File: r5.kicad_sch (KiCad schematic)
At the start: 80 parts, among them SW10 SW_SPDT, SW60 SW_SPDT, SW70 SW_SPDT, SW80 SW_SPDT, U10 LMZ22005, U20 DRV8871DDA, U21 DRV8871DDA, U22 DRV8871DDA, U23 DRV8871DDA, U24 DRV8871DDA, U25 DRV8871DDA, U50 PI22, U60 PCA9685PW, U70 74HC540, U71 74HC540, U80 Pico, X10 Conn_01x02, X11 Conn_01x02, X12 Conn_01x02, X20 Conn_01x06, X21 Conn_01x06, X22 Conn_01x06, X23 Conn_01x06, X24 Conn_01x06, X25 Conn_01x06, X40 Conn_01x04, X90 3X3HEADER, X91 4X3HEADER, X92 SDD1309, X93 GY-BNO08X

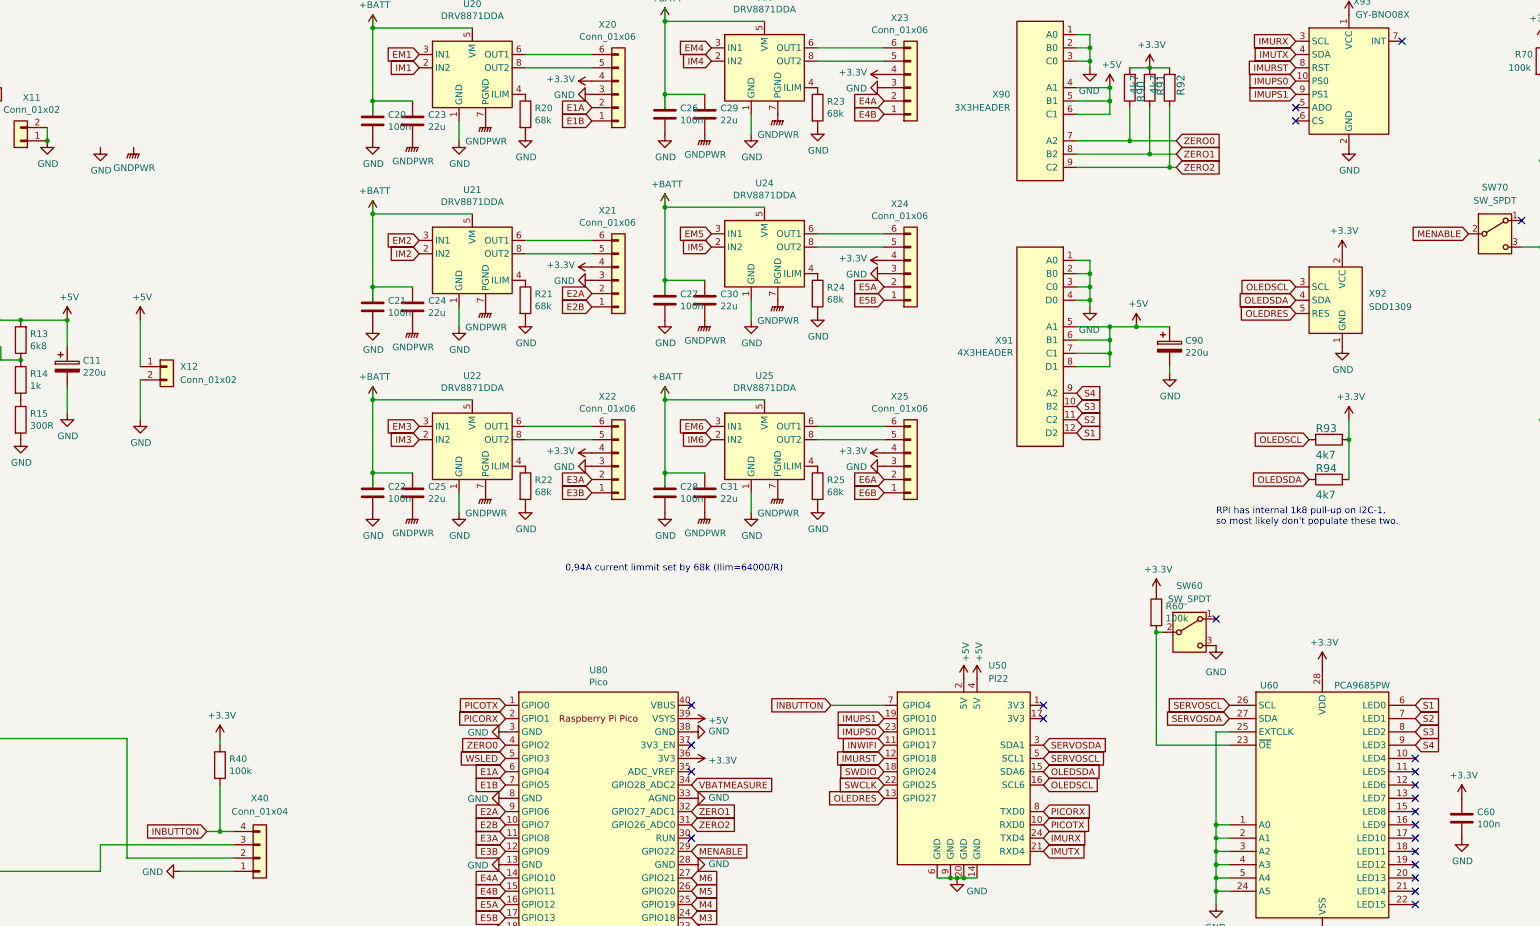
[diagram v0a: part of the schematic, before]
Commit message: routing continued
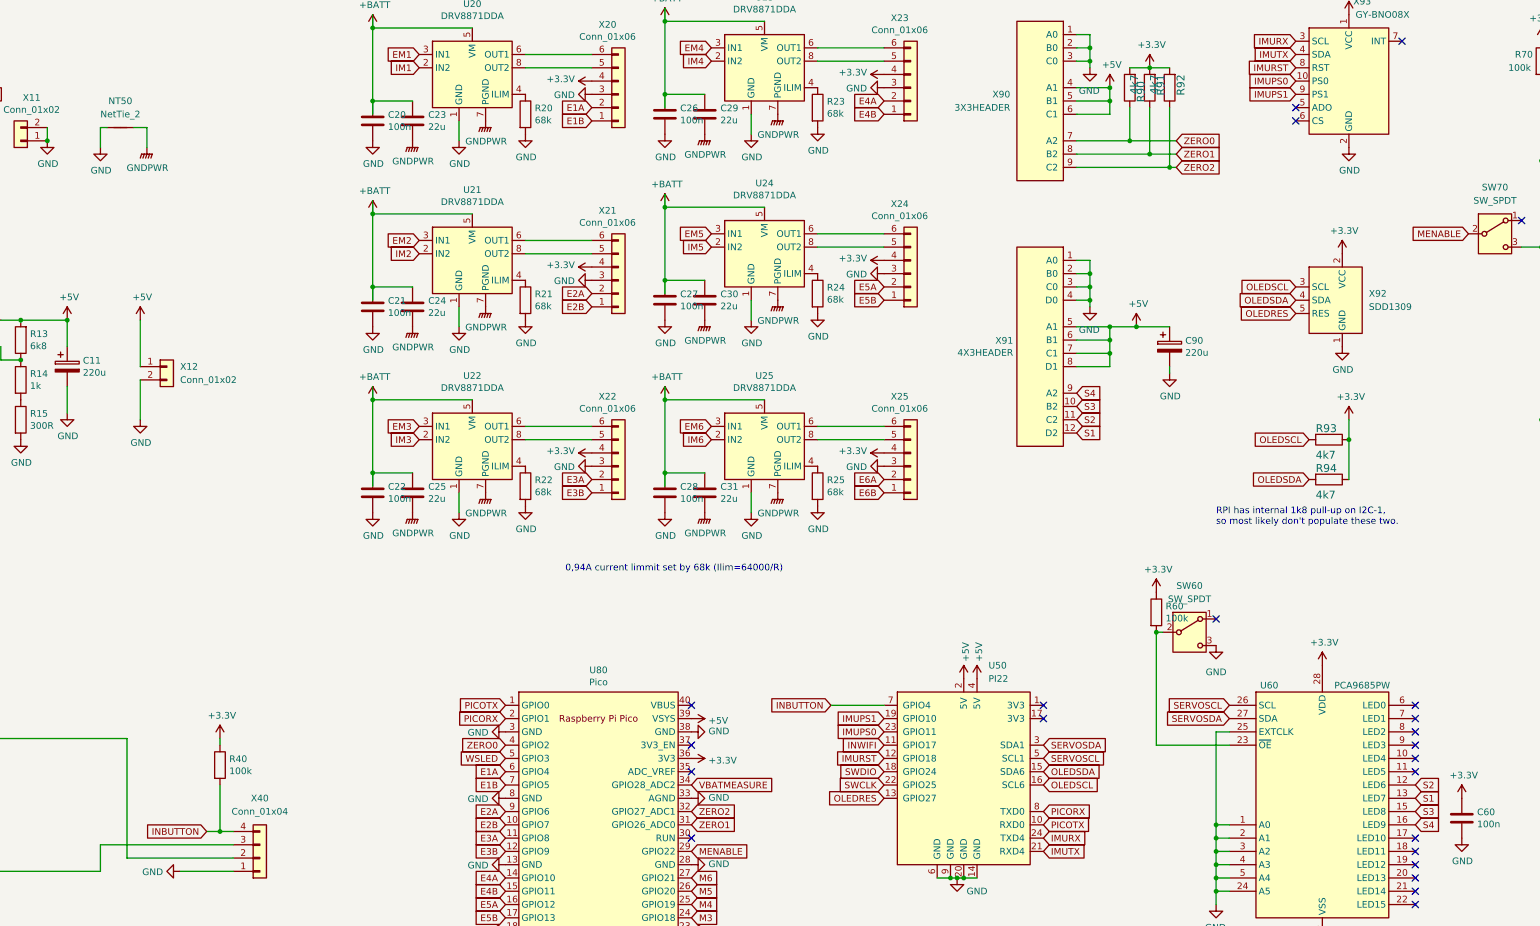
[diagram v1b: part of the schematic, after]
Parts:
- added NT50: NetTie_2, NetTie:NetTie-2_SMD_Pad2.0mm, symbol Device:NetTie_2
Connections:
- net GND: now also NT50.1
- net GNDPWR: now also NT50.2
- net S1: now also U60.13 (LED7); no longer U60.6 (LED0)
- net S2: now also U60.12 (LED6); no longer U60.7 (LED1)
- net S3: now also U60.15 (LED8); no longer U60.8 (LED2)
- net S4: now also U60.16 (LED9); no longer U60.9 (LED3)
- net ZERO1: now also U80.31 (GPIO26_ADC0); no longer U80.32 (GPIO27_ADC1)
- net ZERO2: now also U80.32 (GPIO27_ADC1); no longer U80.31 (GPIO26_ADC0)
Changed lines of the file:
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@@
   )
   (no_connect (at 278.13 175.26))
-  (no_connect (at 349.25 193.04))
+  (no_connect (at 349.25 177.8))
   (no_connect (at 58.42 109.22))
   (no_connect (at 410.21 58.42))
-  (no_connect (at 349.25 190.5))
+  (no_connect (at 349.25 172.72))
   (no_connect (at 210.82 185.42))
   (no_connect (at 349.25 200.66))
@@
   (no_connect (at 326.39 60.96))
   (no_connect (at 410.21 60.96))
-  (no_connect (at 349.25 187.96))
+  (no_connect (at 349.25 175.26))
   (no_connect (at 349.25 205.74))
   (no_connect (at 410.21 113.03))
@@
   (no_connect (at 45.72 107.95))
   (no_connect (at 210.82 198.12))
-  (no_connect (at 349.25 195.58))
+  (no_connect (at 349.25 180.34))
   (no_connect (at 349.25 210.82))
   (no_connect (at 326.39 58.42))
@@
     (stroke (width 0) (type default))
   )
+  (wire (pts (xy 97.79 62.23) (xy 99.06 62.23))
+    (stroke (width 0) (type default))
+  )
   (wire (pts (xy 294.64 50.8) (xy 298.45 50.8))
     (stroke (width 0) (type default))
@@
     (stroke (width 0) (type default))
   )
+  (wire (pts (xy 97.79 66.04) (xy 97.79 62.23))
+    (stroke (width 0) (type default))
+  )
   (wire (pts (xy 149.86 78.74) (xy 149.86 92.71))
     (stroke (width 0) (type default))
@@
     (stroke (width 0) (type default))
   )
+  (wire (pts (xy 104.14 62.23) (xy 106.68 62.23))
+    (stroke (width 0) (type default))
+  )
   (wire (pts (xy 284.48 67.31) (xy 298.45 67.31))
     (stroke (width 0) (type default))
@@
     (stroke (width 0) (type default))
   )
+  (wire (pts (xy 106.68 62.23) (xy 106.68 66.04))
+    (stroke (width 0) (type default))
+  )
   (wire (pts (xy 290.83 102.87) (xy 290.83 100.33))
     (stroke (width 0) (type default))
@@
     )
   )
-  (global_label "S4" (shape input) (at 349.25 180.34 0)
+  (global_label "S4" (shape input) (at 349.25 195.58 0)
     (effects (font (size 1.27 1.27)) (justify left))
-    (property "Intersheetrefs" "${INTERSHEET_REFS}" (at 349.25 180.34 0)
+    (property "Intersheetrefs" "${INTERSHEET_REFS}" (at 349.25 195.58 0)
       (effects (font (size 1.27 1.27)) hide)
     )
@@
     )
   )
-  (global_label "ZERO2" (shape input) (at 210.82 195.58 0) (fields_autoplaced)
+  (global_label "ZERO2" (shape input) (at 210.82 193.04 0) (fields_autoplaced)
     (effects (font (size 1.27 1.27)) (justify left))
-    (property "Intersheetrefs" "${INTERSHEET_REFS}" (at 219.3195 195.58 0)
+    (property "Intersheetrefs" "${INTERSHEET_REFS}" (at 219.3195 193.04 0)
       (effects (font (size 1.27 1.27)) (justify left) hide)
     )
@@
     )
   )
-  (global_label "S1" (shape input) (at 349.25 172.72 0)
+  (global_label "S1" (shape input) (at 349.25 190.5 0)
     (effects (font (size 1.27 1.27)) (justify left))
-    (property "Intersheetrefs" "${INTERSHEET_REFS}" (at 349.25 172.72 0)
+    (property "Intersheetrefs" "${INTERSHEET_REFS}" (at 349.25 190.5 0)
       (effects (font (size 1.27 1.27)) hide)
     )
@@
     )
   )
-  (global_label "ZERO1" (shape input) (at 210.82 193.04 0) (fields_autoplaced)
+  (global_label "ZERO1" (shape input) (at 210.82 195.58 0) (fields_autoplaced)
     (effects (font (size 1.27 1.27)) (justify left))
-    (property "Intersheetrefs" "${INTERSHEET_REFS}" (at 219.3195 193.04 0)
+    (property "Intersheetrefs" "${INTERSHEET_REFS}" (at 219.3195 195.58 0)
       (effects (font (size 1.27 1.27)) (justify left) hide)
     )
   )
-  (global_label "S2" (shape input) (at 349.25 175.26 0)
+  (global_label "S2" (shape input) (at 349.25 187.96 0)
     (effects (font (size 1.27 1.27)) (justify left))
-    (property "Intersheetrefs" "${INTERSHEET_REFS}" (at 349.25 175.26 0)
+    (property "Intersheetrefs" "${INTERSHEET_REFS}" (at 349.25 187.96 0)
       (effects (font (size 1.27 1.27)) hide)
     )
   )
-  (global_label "S3" (shape input) (at 349.25 177.8 0)
+  (global_label "S3" (shape input) (at 349.25 193.04 0)
     (effects (font (size 1.27 1.27)) (justify left))
-    (property "Intersheetrefs" "${INTERSHEET_REFS}" (at 349.25 177.8 0)
+    (property "Intersheetrefs" "${INTERSHEET_REFS}" (at 349.25 193.04 0)
       (effects (font (size 1.27 1.27)) hide)
     )
@@
     )
   )
-  (symbol (lib_id "power:GNDPWR") (at 104.14 66.04 0) (unit 1)
+  (symbol (lib_id "power:GNDPWR") (at 106.68 66.04 0) (unit 1)
     (in_bom yes) (on_board yes) (dnp no)
-    (property "Reference" "#PWR0218" (at 104.14 71.12 0)
+    (property "Reference" "#PWR0218" (at 106.68 71.12 0)
       (effects (font (size 1.27 1.27)) hide)
     )
-    (property "Value" "GNDPWR" (at 104.2416 69.9516 0)
+    (property "Value" "GNDPWR" (at 106.7816 69.9516 0)
       (effects (font (size 1.27 1.27)))
     )
-    (property "Footprint" "" (at 104.14 67.31 0)
+    (property "Footprint" "" (at 106.68 67.31 0)
       (effects (font (size 1.27 1.27)) hide)
     )
-    (property "Datasheet" "" (at 104.14 67.31 0)
+    (property "Datasheet" "" (at 106.68 67.31 0)
       (effects (font (size 1.27 1.27)) hide)
     )
@@
         )
       )
+    )
+  )
+  (symbol (lib_id "Device:NetTie_2") (at 101.6 62.23 0) (unit 1)
+    (in_bom no) (on_board yes) (dnp no) (fields_autoplaced)
+    (property "Reference" "NT50" (at 101.6 57.15 0)
+      (effects (font (size 1.27 1.27)))
+    )
+    (property "Value" "NetTie_2" (at 101.6 59.69 0)
+      (effects (font (size 1.27 1.27)))
+    )
+    (property "Footprint" "NetTie:NetTie-2_SMD_Pad2.0mm" (at 101.6 62.23 0)
+      (effects (font (size 1.27 1.27)) hide)
+    )
+    (property "Datasheet" "~" (at 101.6 62.23 0)
+      (effects (font (size 1.27 1.27)) hide)
+    )
+    (pin "2")
+    (pin "1")
+    (instances
+      (project "r5"
+        (path "/7141c11d-0c81-438d-ad8c-6c0ffa292856"
+          (reference "NT50") (unit 1)
+        )
+      )
